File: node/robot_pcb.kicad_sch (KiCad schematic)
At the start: 25 parts, among them J1 Conn_01x19_Female, J2 Conn_01x19_Female, J3 esp32Cam, M1 Motor_DC, M5 Motor_DC, Q1 IRF4905, Q2 IRFZ44NPBF, Q3 IRF4905, Q4 IRFZ44NPBF, Q5 IRF4905, Q6 IRFZ44NPBF, Q7 IRF4905, Q8 IRFZ44NPBF, U1 4N25, U2 4N25, U3 4N25, U4 4N25

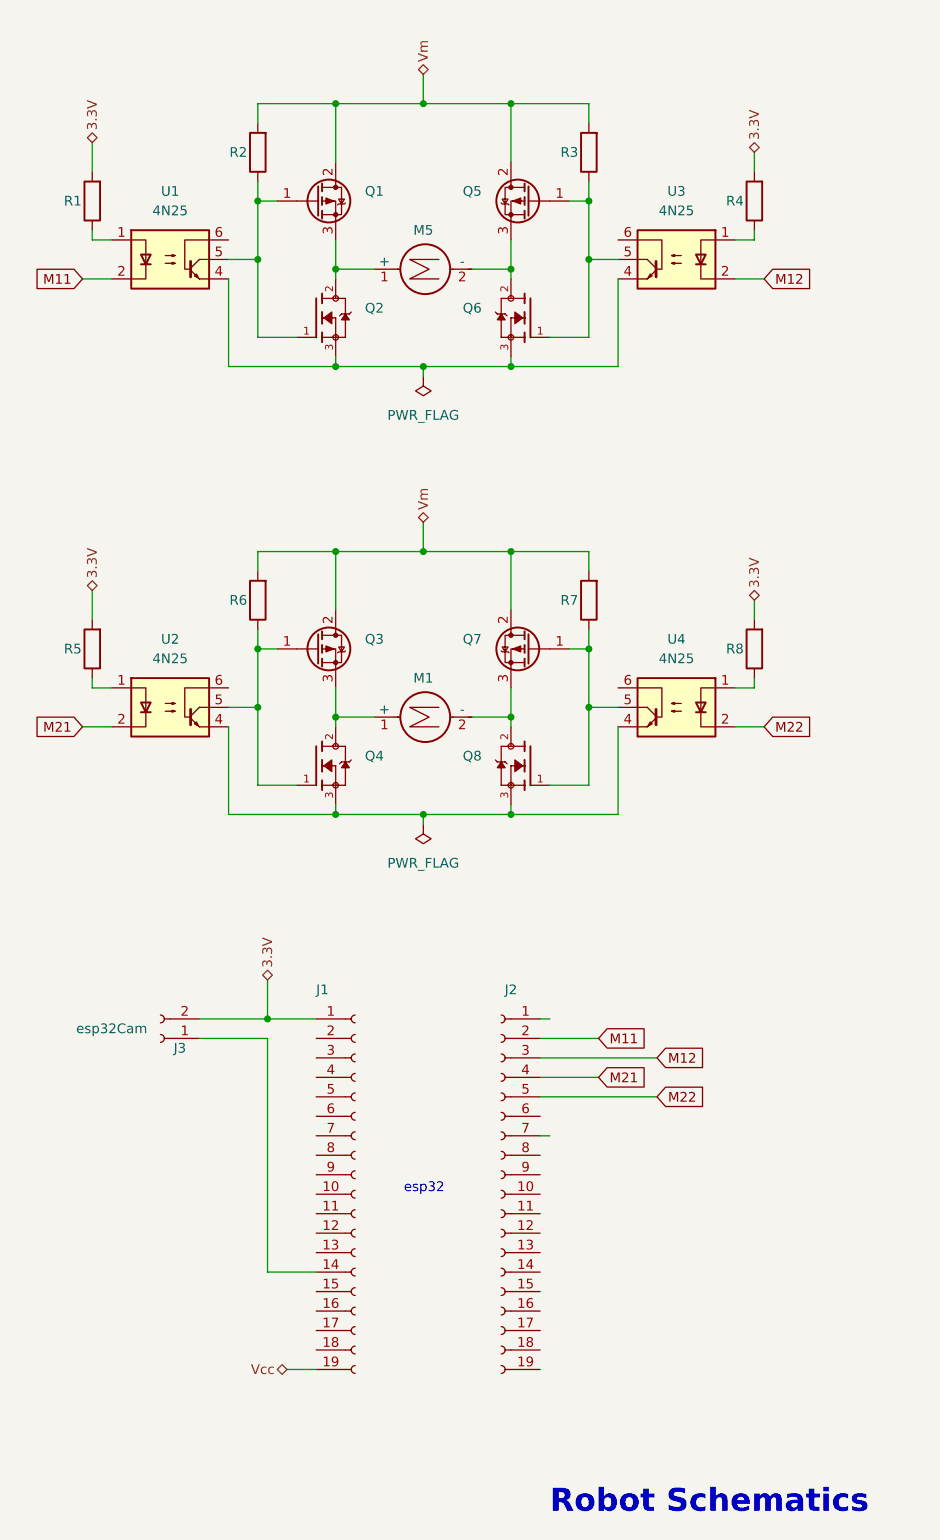
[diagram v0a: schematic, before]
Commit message: pcb design complete
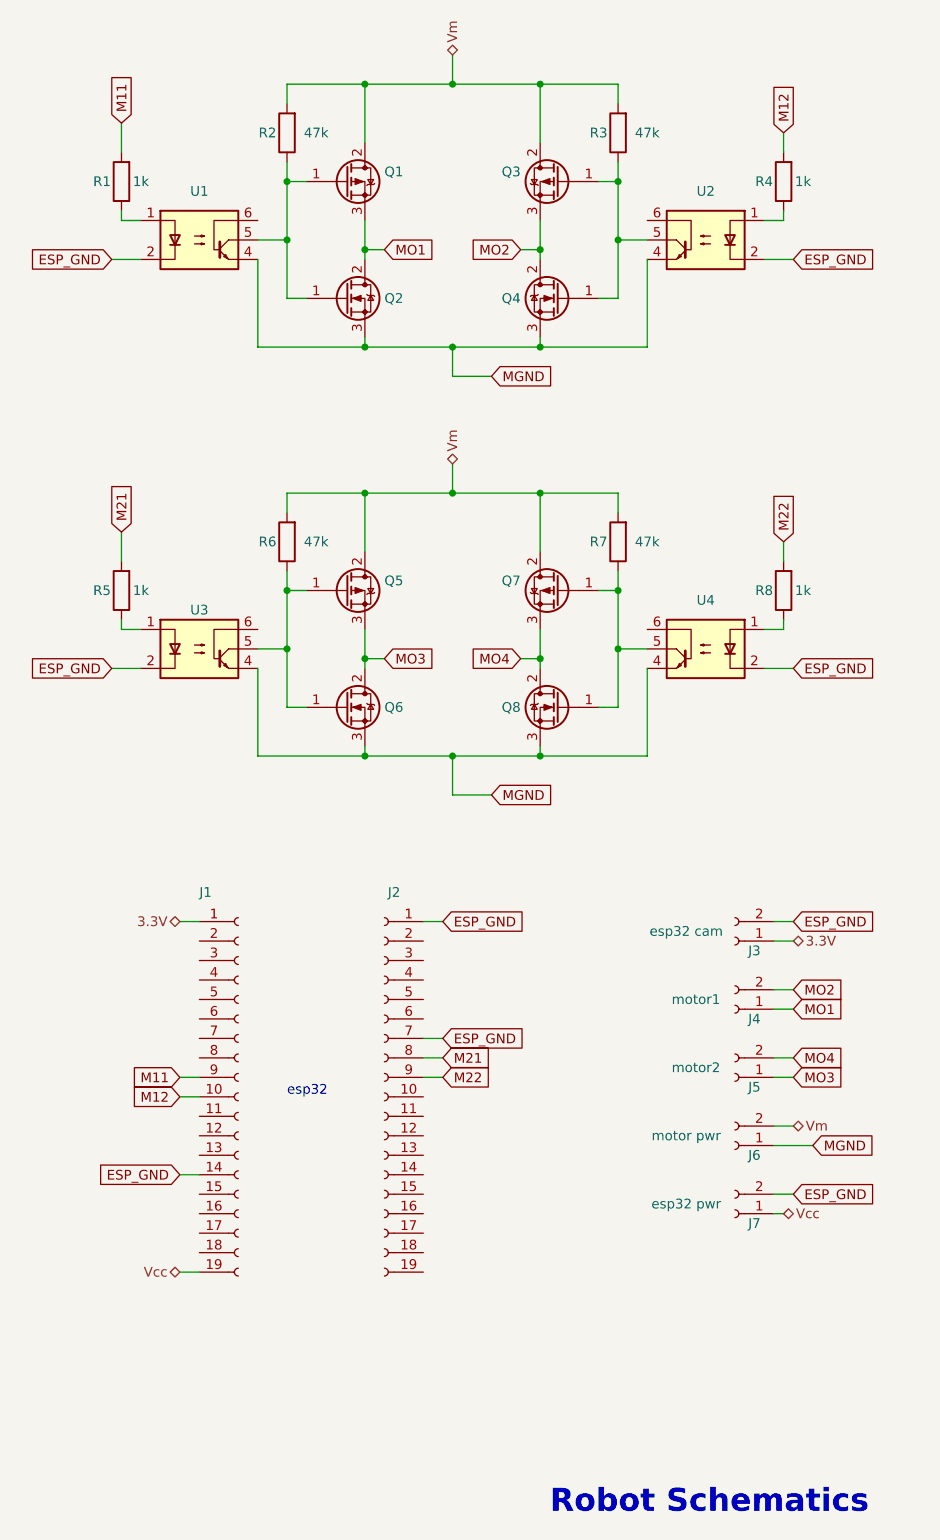
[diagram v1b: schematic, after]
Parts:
- removed M1, M5: Motor_DC, symbol Motor:Motor_DC
- removed Q2, Q4, Q6, Q8: IRFZ44NPBF, TO254P1016X419X2286-3, symbol IRFZ44NPBF:IRFZ44NPBF
- removed Q3: IRF4905, Package_TO_SOT_THT:TO-220-3_Vertical, symbol Transistor_FET:IRF4905
- removed U2: 4N25, Package_DIP:DIP-6_W7.62mm, symbol Isolator:4N25
- added J4: motor1, Connector_PinHeader_2.54mm:PinHeader_1x02_P2.54mm_Vertical, symbol Connector:Conn_01x02_Female
- added J5: motor2, Connector_PinHeader_2.54mm:PinHeader_1x02_P2.54mm_Vertical, symbol Connector:Conn_01x02_Female
- added J6: motor pwr, Connector_PinHeader_2.54mm:PinHeader_1x02_P2.54mm_Vertical, symbol Connector:Conn_01x02_Female
- added J7: esp32 pwr, Connector_PinHeader_2.54mm:PinHeader_1x02_P2.54mm_Vertical, symbol Connector:Conn_01x02_Female
- added Q2, Q4, Q6, Q8: Q_NMOS_GDS, Downloads:SOIC127P490X600X175-8N, symbol Device:Q_NMOS_GDS
- added Q5: IRF4905, Downloads:SOIC127P490X600X175-8N, symbol Transistor_FET:IRF4905
- added U3: 4N25, Package_DIP:DIP-6_W7.62mm, symbol Isolator:4N25
- J3: value esp32Cam -> esp32 cam
- Q1, Q7: footprint Package_TO_SOT_THT:TO-220-3_Vertical -> Downloads:SOIC127P490X600X175-8N
- Q3: renamed from Q5; footprint Package_TO_SOT_THT:TO-220-3_Vertical -> Downloads:SOIC127P490X600X175-8N
- R1, R2, R3, R4, R5, R6, R7, R8: footprint Resistor_THT:R_Axial_DIN0614_L14.3mm_D5.7mm_P15.24mm_Horizontal -> Resistor_SMD:R_0201_0603Metric_Pad0.64x0.40mm_HandSolder
- renumbered U3 to U2
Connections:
- net 3.3V: now also J3.1 (Pin_1); no longer J3.2 (Pin_2), R1.2, R4.2, R5.2, R8.2
- net M11: now also J1.9 (Pin_9), R1.2; no longer J2.2 (Pin_2), U1.2
- net M12: now also J1.10 (Pin_10), R4.2; no longer J2.3 (Pin_3), U2.2
- net M21: now also J2.8 (Pin_8), R5.2; no longer J2.4 (Pin_4)
- net M22: now also J2.9 (Pin_9), R8.2; no longer J2.5 (Pin_5), U4.2
- net Vcc: now also J7.1 (Pin_1)
- net Vm: now also J6.2 (Pin_2), Q5.2 (D)
- net at Q7.1 (G), R7.1, U4.5: now also Q8.1 (G)
- net MO4: now reaches Q7.3 (S)
- net MO4: now also J5.2 (Pin_2), Q8.2 (D)
- net MGND: now reaches U4.4
- net MGND: now also U1.4, U2.4, J6.1 (Pin_1), Q2.3 (S), Q4.3 (S), Q6.3 (S), Q8.3 (S), U3.4
- net at Q1.1 (G), R2.1, U1.5: now also Q2.1 (G)
- net at Q3.1 (G), R3.1, U2.5: now also Q4.1 (G)
- net MO2: now reaches Q3.3 (S)
- net MO2: now also J4.2 (Pin_2), Q4.2 (D)
- net at R6.1: now also Q5.1 (G), Q6.1 (G), U3.5
- net at R5.1: now also U3.1
- net MO1: now reaches Q1.3 (S)
- net MO1: now also J4.1 (Pin_1), Q2.2 (D)
- net ESP_GND: now reaches J1.14 (Pin_14)
- net ESP_GND: now also J2.1 (Pin_1), J2.7 (Pin_7), J3.2 (Pin_2), U1.2, U2.2, U4.2, J7.2 (Pin_2), U3.2; no longer J3.1 (Pin_1)
- new net MO3: J5.1 (Pin_1), Q5.3 (S), Q6.2 (D)
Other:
- moved on the sheet: J1, J2, Q1, Q3, R1, R2, U1, U2
